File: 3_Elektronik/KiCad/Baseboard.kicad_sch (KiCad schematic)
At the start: 75 parts, among them J1 Conn_02x10_Odd_Even, J2 Conn_02x10_Odd_Even, J3 Conn_02x10_Odd_Even, J4 Conn_02x10_Odd_Even, J5 Conn_01x04_Pin, J6 693072010801, J7 629722000214, Q1 2N7002K, Q2 DMP3099L, SW2 434331013822, SW3 434331013822, U1 LSM6DSV320XTR, U2 TPS7B8601QDDARQ1, U3 TCAN334, U4 ESP32-S3-WROOM-1, U5 LSM6DSO32XTR, U6 DPS310, U7 LIS3MDL, U8 CH224A

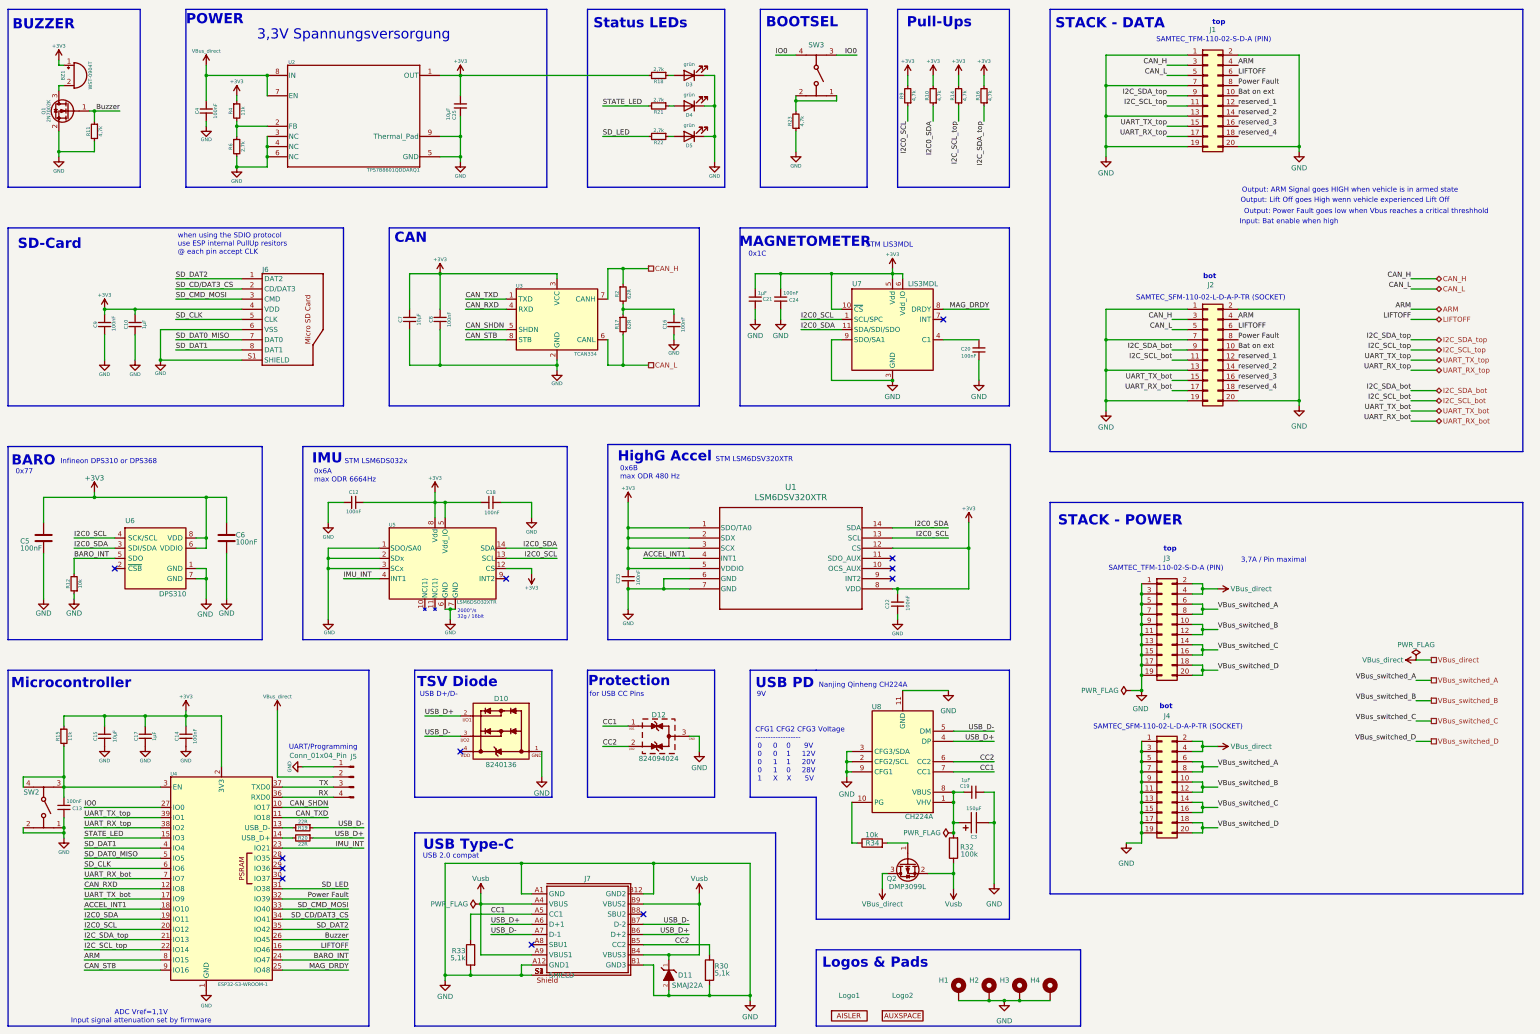
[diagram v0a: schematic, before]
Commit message: style: :art: split schematics into subpages
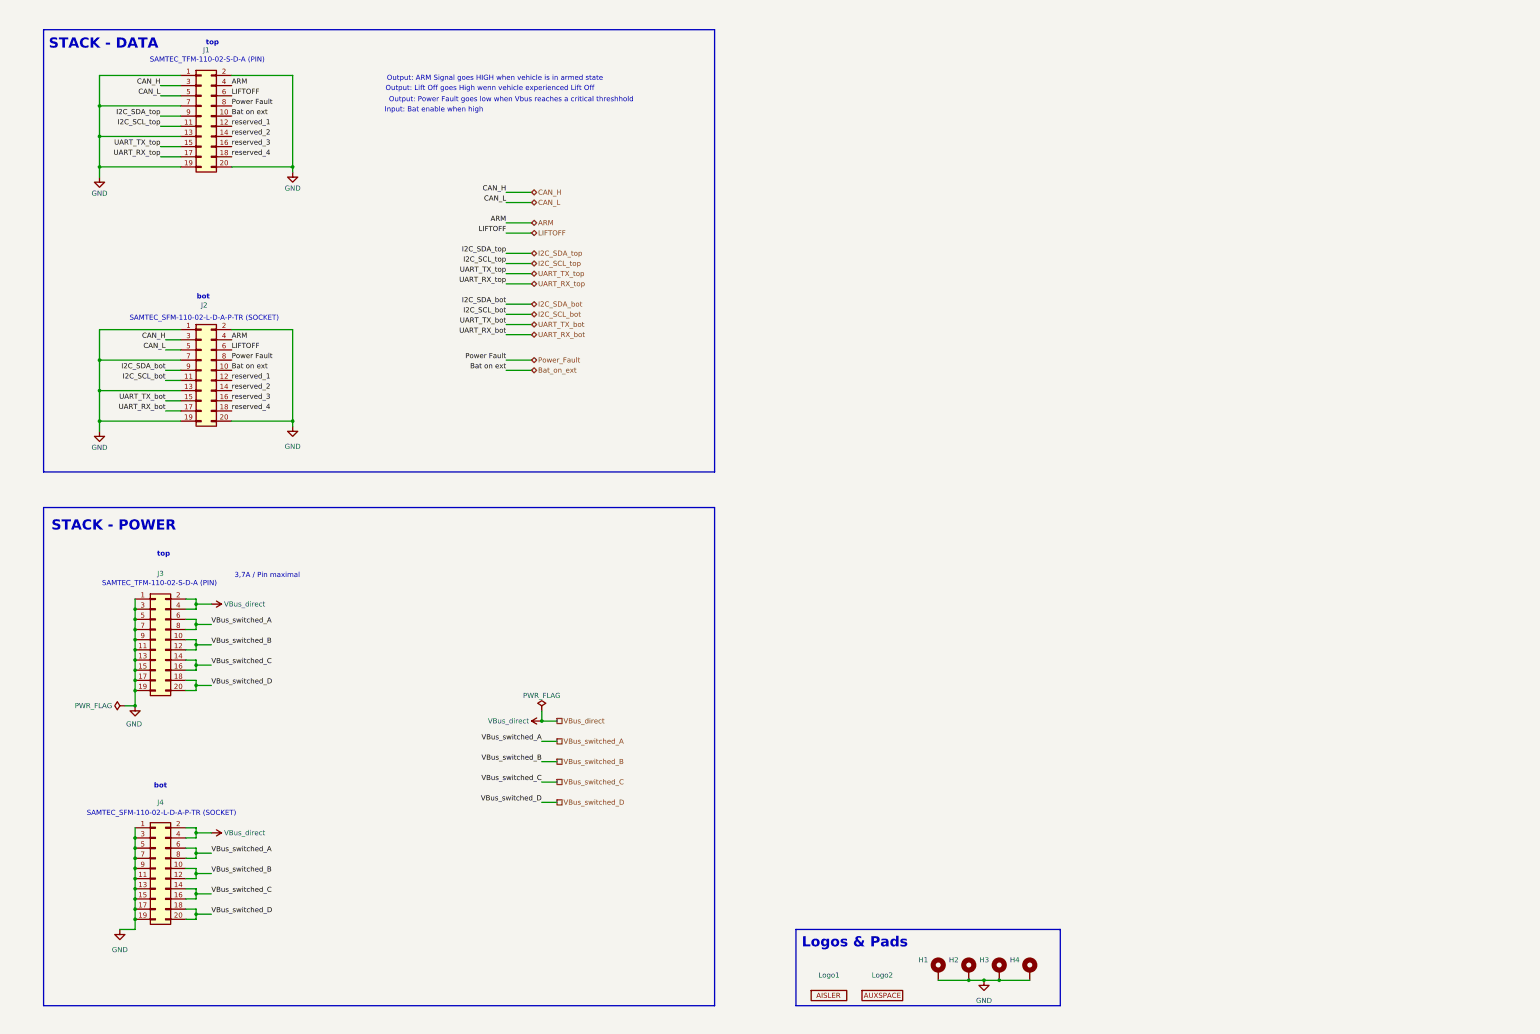
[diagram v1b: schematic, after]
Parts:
- removed BZ1: WST-0904T, AUXSPACE:Buzzer_WST-0906T, symbol Device:Buzzer
- removed C10, C17, C19, C21: 1µF, Capacitor_SMD:C_0603_1608Metric, symbol Device:C_Small
- removed C12, C13, C14, C16, C18, C20, C22, C23, C24, C4, C8, C9: 100nF, Capacitor_SMD:C_0603_1608Metric, symbol Device:C_Small
- removed C15, C25, C7: 10µF, Capacitor_SMD:C_0603_1608Metric, symbol Device:C_Small
- removed C3: 150 µF, AUXSPACE:CP_Wurth_WCAP-ASLL-D6.3L5.5, symbol AUXSPACE:D6.3L5.5_865060243005
- removed C5, C6: 100nF, Capacitor_SMD:C_0603_1608Metric, symbol Device:C
- removed D10: 8240136, AUXSPACE:WE-TVS_SOT143-4L, symbol AUXSPACE:WE-TVS-HS_SOT143-4L_8240136
- removed D11: SMAJ22A, AUXSPACE:WE-TVS_SMAJ22A, symbol AUXSPACE:WE-TVSP_DO-214AC_400W_UNI
- removed D12: 824094024, AUXSPACE:WE-TVS_824094024_SOT23-3L, symbol AUXSPACE:SOT23-3L_824094024
- removed D3, D4, D5: grün, LED_SMD:LED_0603_1608Metric, symbol Device:LED
- removed J5: Conn_01x04_Pin, symbol Connector:Conn_01x04_Pin
- removed J6: 693072010801, AUXSPACE:J_Wurth_WR-CRD_693072010801, symbol AUXSPACE:693072010801
- removed J7: 629722000214, AUXSPACE:J_Wurth_WR-USB_629722000214, symbol AUXSPACE:629722000214
- removed Q1: 2N7002K, Package_TO_SOT_SMD:SOT-23, symbol Transistor_FET:2N7002K
- removed Q2: DMP3099L, Package_TO_SOT_SMD:SOT-23, symbol Transistor_FET:DMP3099L
- removed R10, R11, R14, R16, R23, R9: 4,7k, Resistor_SMD:R_0603_1608Metric, symbol Device:R_Small
- removed R12: 10k, Resistor_SMD:R_0603_1608Metric, symbol Device:R_Small
- removed R15, R4: 11k, Resistor_SMD:R_0603_1608Metric, symbol Device:R_Small
- removed R17, R2: 62R, Resistor_SMD:R_0603_1608Metric, symbol Device:R_Small
- removed R18, R21, R22, R6: 2,7k, Resistor_SMD:R_0603_1608Metric, symbol Device:R_Small
- removed R19, R20: 22R, Resistor_SMD:R_0603_1608Metric, symbol Device:R_Small
- removed R30, R33: 5,1k, Resistor_SMD:R_0603_1608Metric, symbol Device:R
- removed R32: 100k, Resistor_SMD:R_0603_1608Metric, symbol Device:R
- removed R34: 10k, Resistor_SMD:R_0603_1608Metric, symbol Device:R
- removed SW2, SW3: 434331013822, AUXSPACE:SW_Wurth_WS-TASU_434331013822, symbol AUXSPACE:434331013822
- removed U1: LSM6DSV320XTR, AUXSPACE:LGA-14L_2p5X3X0p83_STM, symbol AUXSPACE:LSM6DSV320XTR
- removed U2: TPS7B8601QDDARQ1, AUXSPACE:Texas_R-PDSO-G8_EP2.95x4.9mm_Mask2.4x3.1mm_ThermalVias, symbol AUXSPACE:TPS7B8601QDDARQ1
- removed U3: TCAN334, Package_SO:SOIC-8_3.9x4.9mm_P1.27mm, symbol AUXSPACE:TCAN334
- removed U4: ESP32-S3-WROOM-1, AUXSPACE:ESP32-S3-WROOM-1, symbol AUXSPACE:ESP32-S3-WROOM-1
- removed U5: LSM6DSO32XTR, AUXSPACE:LGA_O32XTR_STM, symbol AUXSPACE:LSM6DSO32XTR
- removed U6: DPS310, AUXSPACE:DPS310, symbol AUXSPACE:DPS310
- removed U7: LIS3MDL, Package_LGA:LGA-12_2x2mm_P0.5mm, symbol Sensor_Magnetic:LIS3MDL
- removed U8: CH224A, AUXSPACE:ESSOP-10-1EP_3.9x5.0mm_P1mm_EP2.1x3.3mm, symbol CH224A:CH224A
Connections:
- net Bat on ext renamed Bat_on_ext
- net Power Fault renamed Power_Fault
- no-connect marks 12 -> 0
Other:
- note removed: "0x1C"
- note removed: "0x6A max ODR 6664Hz"
- note removed: "0x6B max ODR 480 Hz"
- note removed: "0x77"
- note removed: "2000°/s 32g / 16bit"
- note removed: "3,3V Spannungsversorgung"
- note removed: "9V"
- note removed: "ADC Vref=1,1V Input signal attenuation set by firmware"
- note removed: "BARO"
- note removed: "BOOTSEL"
- note removed: "BUZZER"
- note removed: "CAN"
- note removed: "CFG1 CFG2 CFG3 Voltage ------------------ 0 0 0 9V 0 0 1 12V 0 1 1 20V 0 1 0 28V 1 X X 5V"
- note removed: "HighG Accel"
- note removed: "IMU"
- note removed: "Infineon DPS310 or DPS368"
- note removed: "MAGNETOMETER"
- note removed: "Microcontroller"
- note removed: "Nanjing Qinheng CH224A"
- note removed: "POWER"
- note removed: "Protection"
- note removed: "Pull-Ups"
- note removed: "SD-Card"
- note removed: "STM LIS3MDL"
- note removed: "STM LSM6DS032x"
- note removed: "STM LSM6DSV320XTR"
- note removed: "Status LEDs"
- note removed: "TSV Diode"
- note removed: "UART/Programming"
- note removed: "USB 2.0 compat"
- note removed: "USB D+/D-"
- note removed: "USB PD"
- note removed: "USB Type-C"
- note removed: "for USB CC Pins"
- note removed: "when using the SDIO protocol use ESP internal PullUp resitors @ each pin accept CLK"
- moved on the sheet: H1, H2, H3, H4, J1, J2, J3, J4, Logo1, Logo2
